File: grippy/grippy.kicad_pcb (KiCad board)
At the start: 2 copper layers, 60.8 x 35.2 mm, 9 parts, among them J1 Conn_01x08_Socket, SW0 SW_SPST, SW1 SW_SPST, SW2 SW_SPST, SW3 SW_SPST, SW4 SW_SPST, SW5 SW_DPDT_x2, U1 esp32s3-supermini

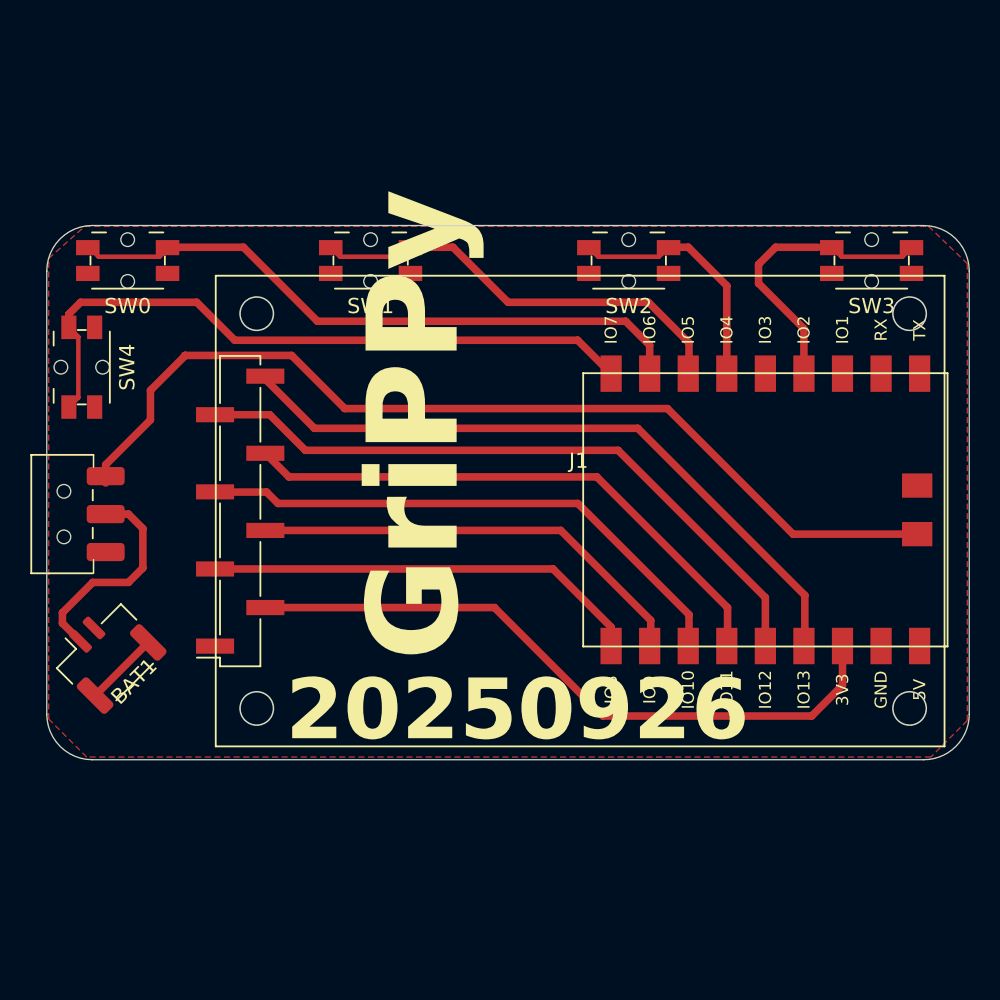
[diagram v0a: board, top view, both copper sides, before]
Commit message: working model
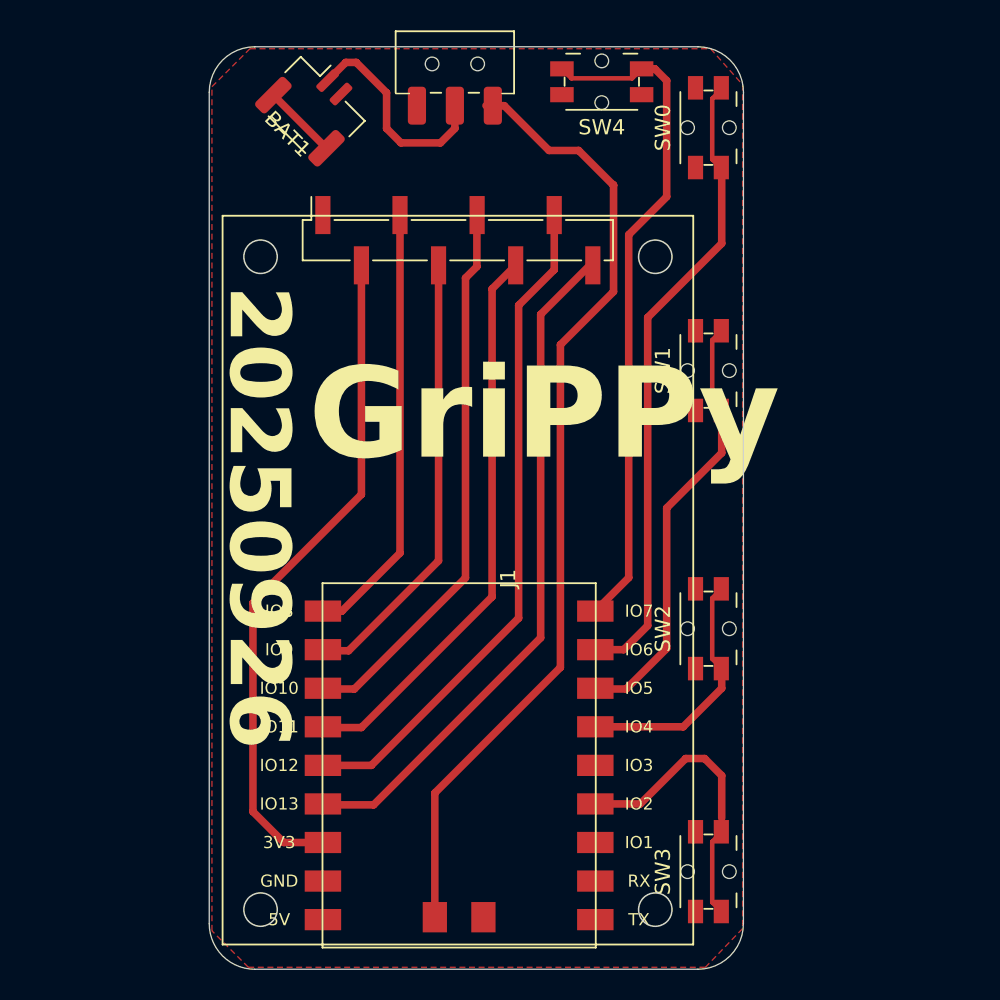
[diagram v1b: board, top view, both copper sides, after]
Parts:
- moved SW3 41.7 mm to (220.4, 109.2), turned to -90 degrees
- moved SW0 39.2 mm to (220.4, 60.2), turned to -90 degrees
- moved SW4 39.1 mm to (213.4, 57.2), turned to 0 degrees
- moved SW5 38.9 mm to (203.8, 56.3), turned to 180 degrees
- moved BAT1 38.5 mm to (194.5, 58.9), turned to -45 degrees
- moved U1 26.3 mm to (204.0, 102.2), turned to 0 degrees
- moved SW2 24.8 mm to (220.4, 93.2), turned to -90 degrees
- moved SW1 23.4 mm to (220.4, 76.2), turned to -90 degrees
- moved J1 9.25 mm to (203.9, 90.0), turned to -90 degrees
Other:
- board size 60.8 x 35.2 mm -> 35.2 x 60.8 mm
